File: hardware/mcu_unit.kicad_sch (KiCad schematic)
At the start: 75 parts, among them J7 61300411121, U10 RP2040, U9 W25Q128JVPIQ, Y1 ABM8-272-T3

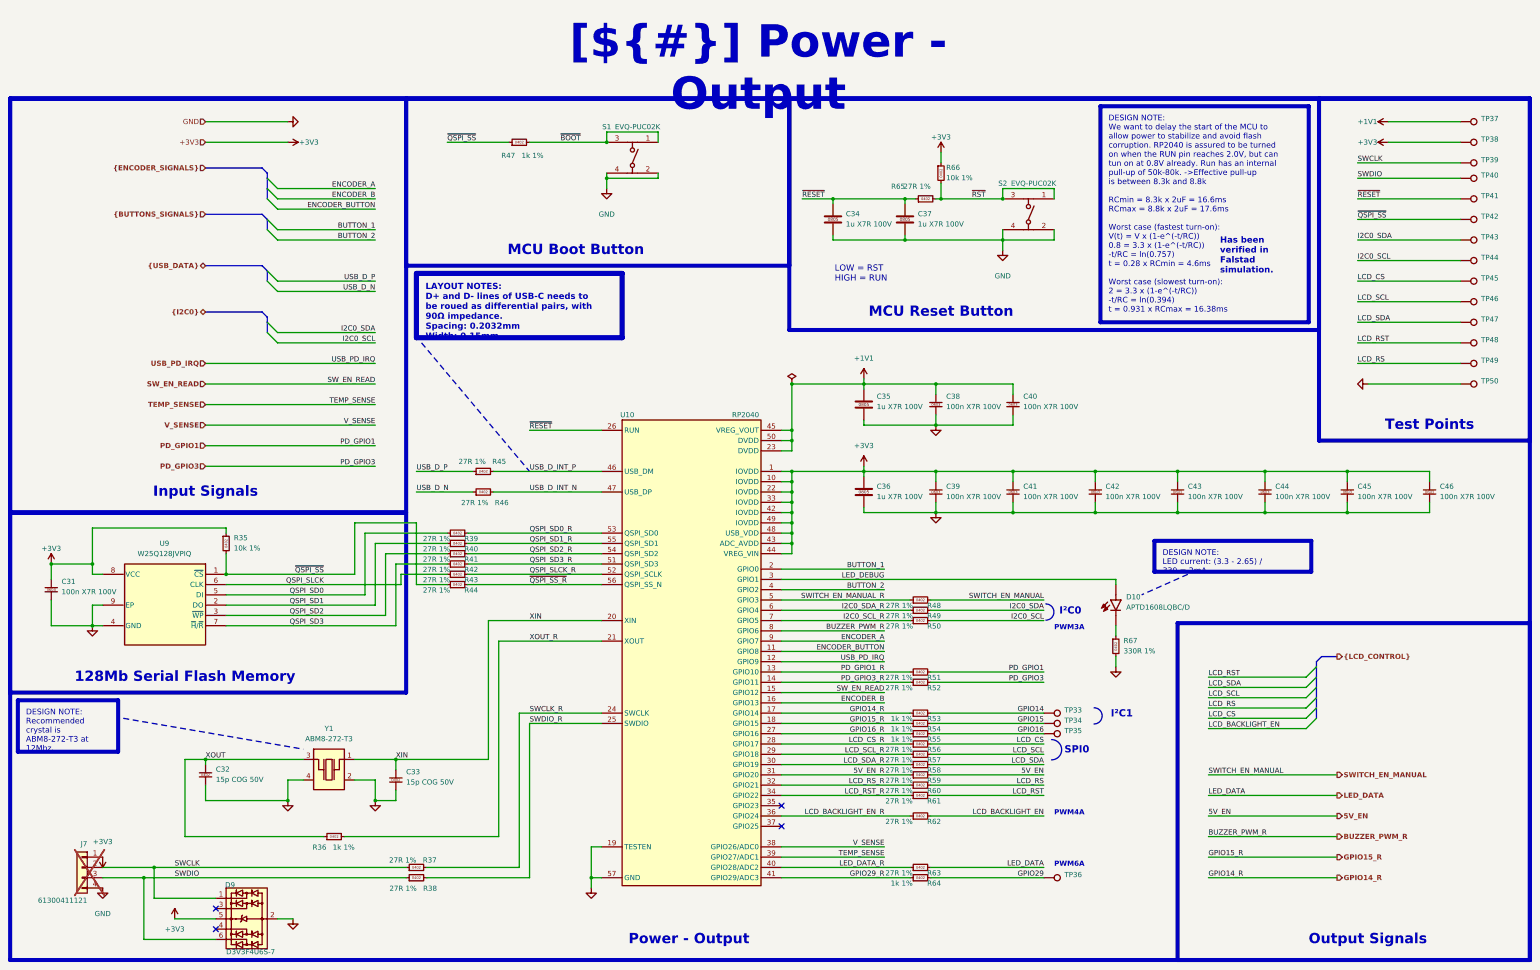
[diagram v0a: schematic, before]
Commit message: Generate hardware documentation
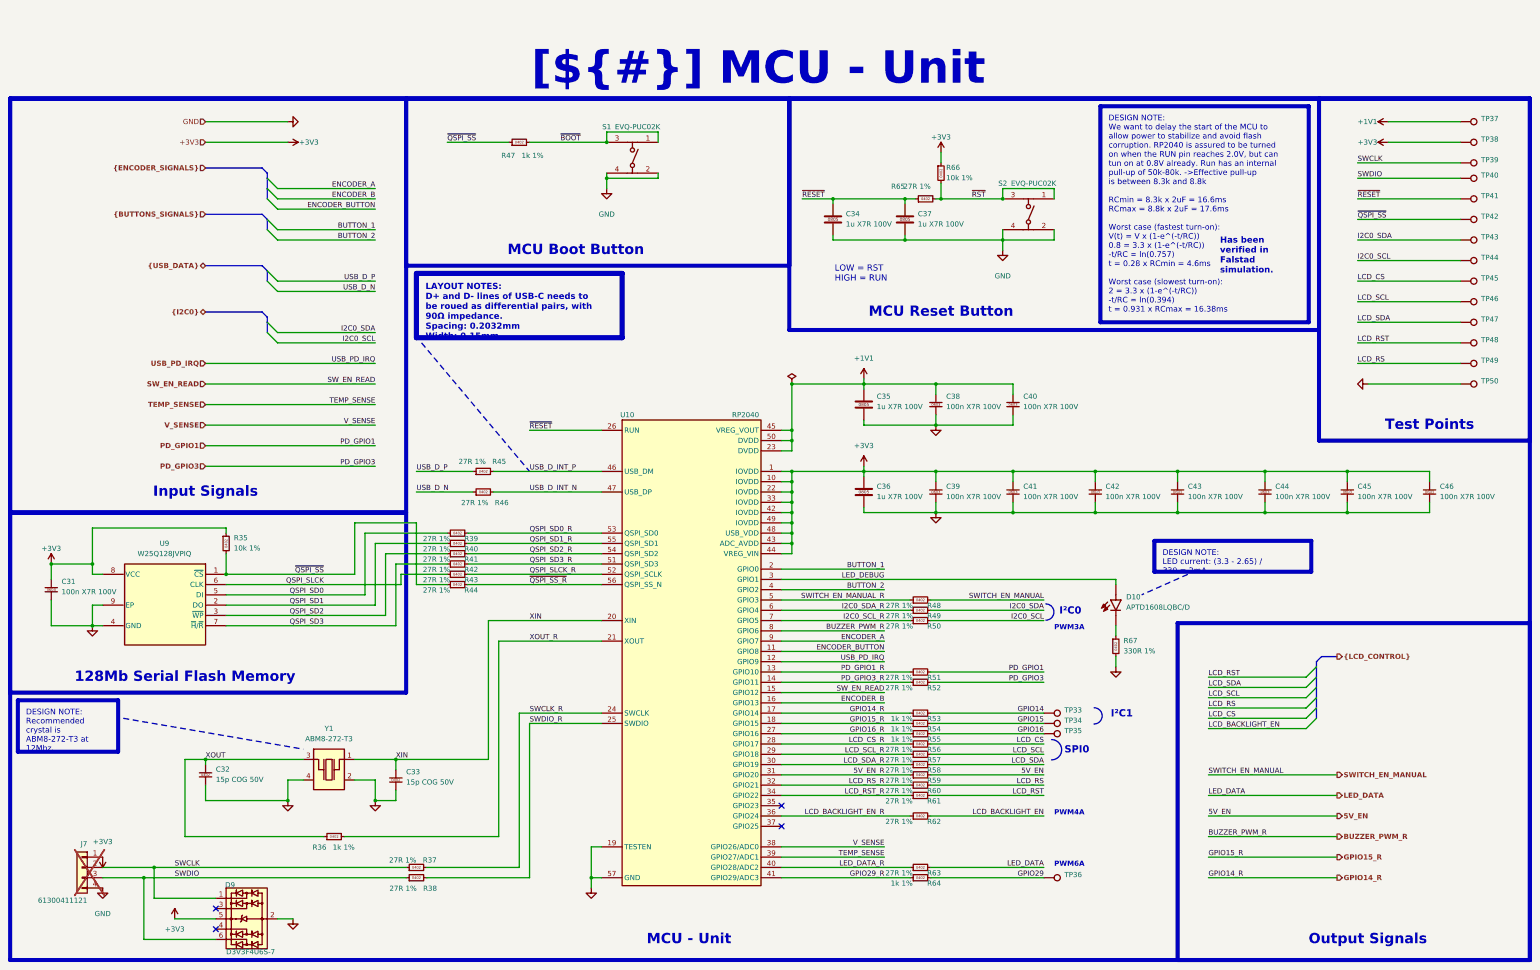
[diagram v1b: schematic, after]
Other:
- title: Power - Output -> MCU - Unit
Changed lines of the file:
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@@
 	(paper "A3")
 	(title_block
-		(title "Power - Output")
+		(title "MCU - Unit")
 		(date "2026-02-27")
 		(rev "${REVISION}")
